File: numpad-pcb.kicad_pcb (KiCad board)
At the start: 2 copper layers, 62 parts, among them J1 AVR-ISP-6, SW1 SW_Push, SW10 7/home, SW11 4/left, SW12 8/up, SW13 5, SW14 9/pgup, SW15 6/right, SW16 +, SW18 1/end, SW19 0/insert, SW2 ESC, SW20 2/down, SW22 3/pgdn, SW23 ./delete, SW24 ENTER, SW3 TAB, SW4 BACKSPACE, SW5 FN, SW6 NUM_LOCK, SW7 /, SW8 *, SW9 -, U1 ATmega32U4-A, Y1 Crystal_GND24_Small

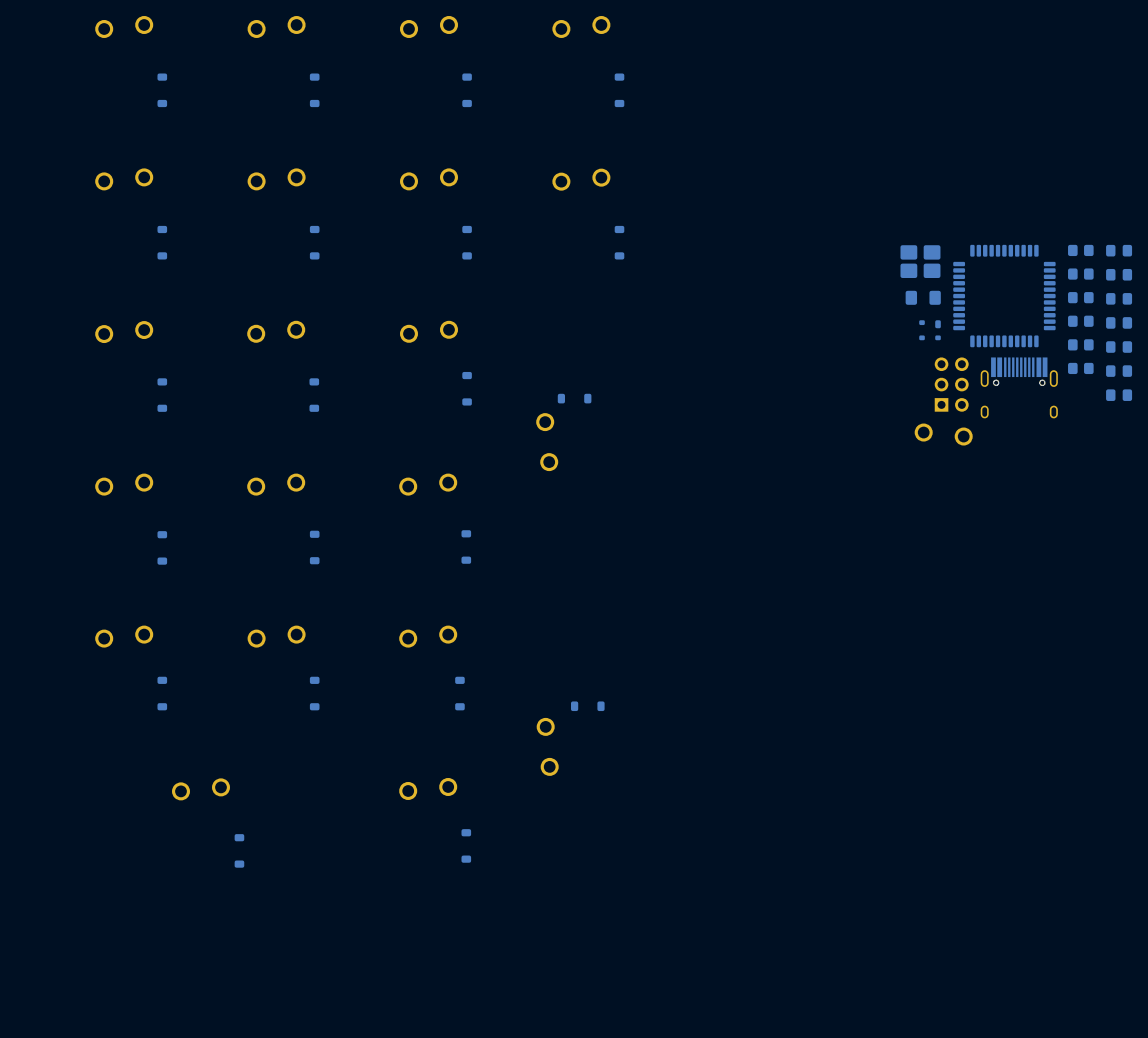
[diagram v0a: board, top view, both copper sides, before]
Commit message: Initial layout of PCB components
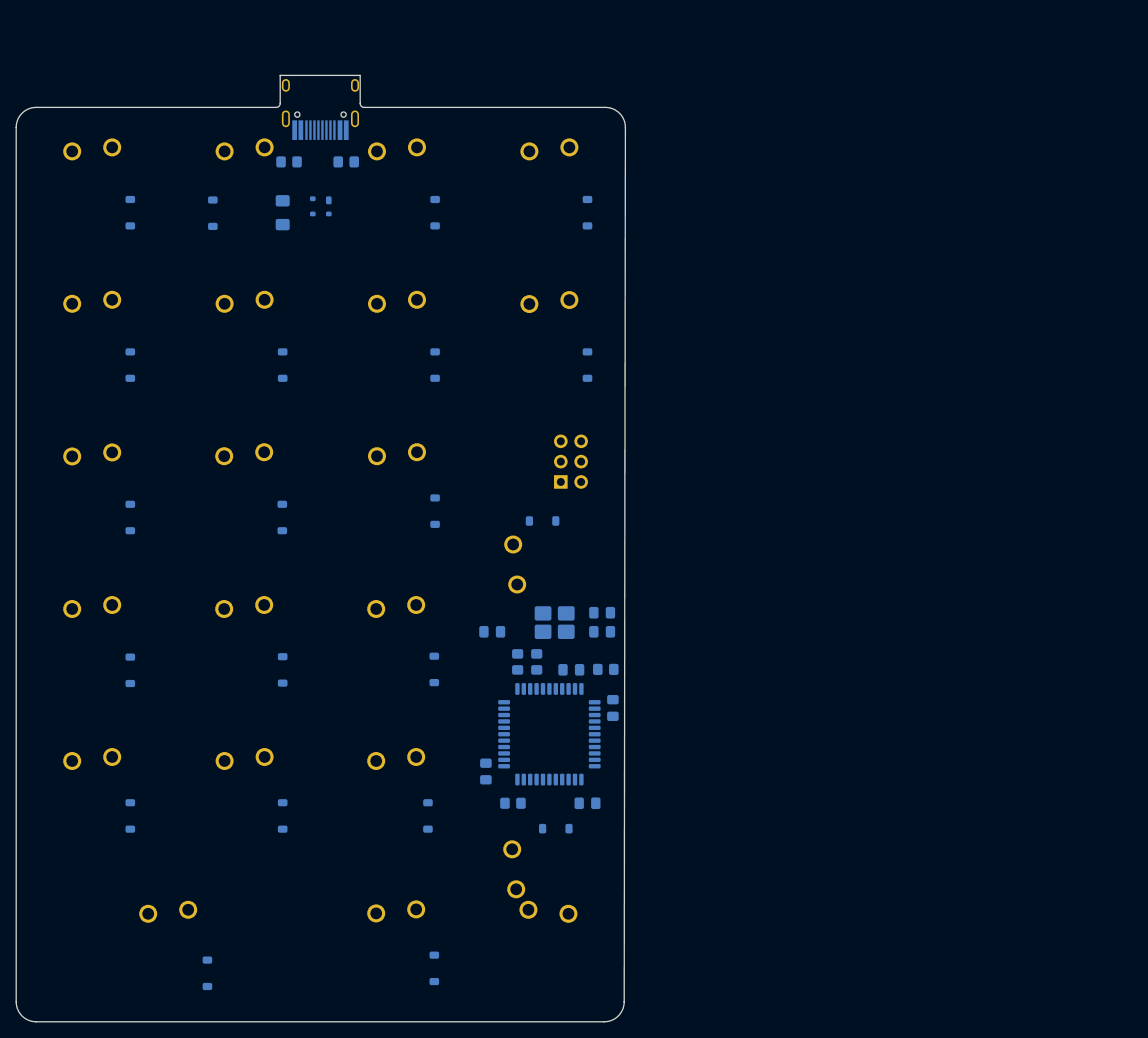
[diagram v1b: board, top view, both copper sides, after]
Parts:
- moved R6 102.3 mm to (84.1, 51.8)
- moved R1 99.1 mm to (112.1, 132.0)
- moved C3 98.8 mm to (108.7, 128.0), turned to 90 degrees
- moved USB1 98.7 mm to (88.0, 39.6), turned to 0 degrees
- moved C1 95.8 mm to (121.4, 132.0)
- moved R5 94.6 mm to (91.2, 51.8)
- moved C4 87.3 mm to (109.5, 110.5)
- moved R3 83.8 mm to (112.7, 114.3), turned to -90 degrees
- moved R2 83.5 mm to (115.1, 114.3), turned to -90 degrees
- moved C2 83.3 mm to (124.6, 120.1), turned to -90 degrees
- moved F1 80.8 mm to (83.3, 58.2), turned to -90 degrees
- moved C5 79.5 mm to (119.4, 115.3)
- moved U1 79.0 mm to (116.7, 123.4), turned to -90 degrees
- moved D1 77.7 mm to (88.1, 57.4)
- moved SW1 77.5 mm to (116.5, 149.8)
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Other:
- board outline added: 76.2 x 118.3 mm
